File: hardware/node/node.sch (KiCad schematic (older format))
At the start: 64 parts, among them J1 BOOT0_Jumper, J2 FTDI, J3 SMA Female, J4 2 x AA, J5 SWD, Q1 Si2323DDS, SW1 TVCM04N016BB, U1 RFM69HW, U2 SHTC3, U3 AT25DF512C, U4 STM32L031K6Tx, Y1 32.768K-CFPX217

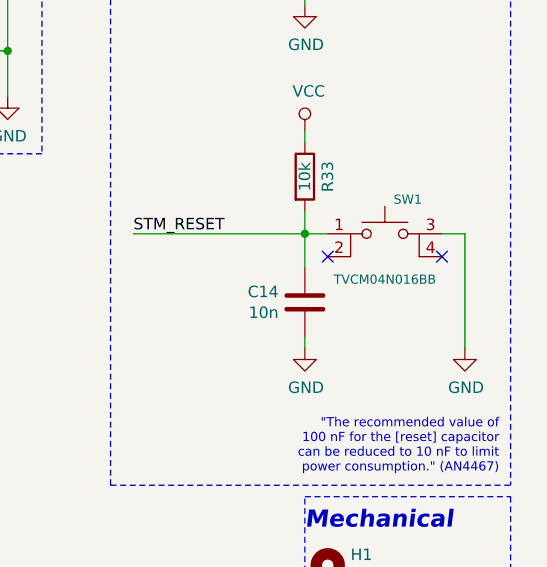
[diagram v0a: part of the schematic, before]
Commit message: Changed switch
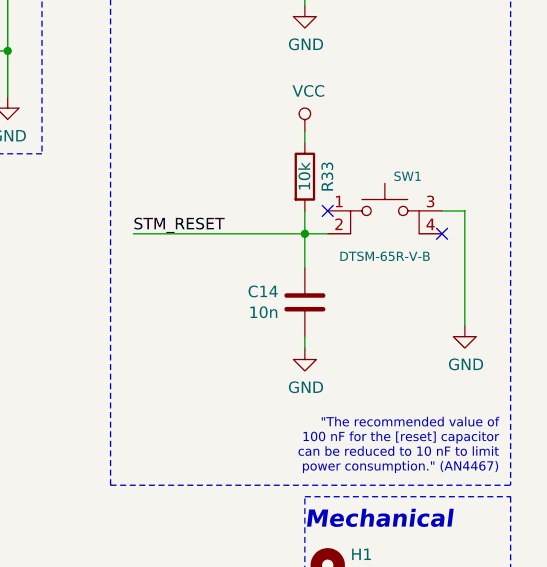
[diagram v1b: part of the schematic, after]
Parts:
- J2: footprint Connector_PinHeader_2.54mm:PinHeader_1x06_P2.54mm_Vertical -> Connector_PinHeader_2.54mm:PinHeader_1x06_P2.54mm_Horizontal
- SW1: value TVCM04N016BB -> DTSM-65R-V-B; footprint humidity:SW_TVCM04-N -> humidity:SW_SPST_DTSM-6
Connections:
- net STM_RESET: now also SW1.2; no longer SW1.1
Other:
- moved on the sheet: SW1
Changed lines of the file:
@@
 L power:GND #PWR032
 U 1 1 5CE4C513
-P 11000 3150
-F 0 "#PWR032" H 11000 2900 50  0001 C CNN
-F 1 "GND" H 11005 2977 50  0000 C CNN
-F 2 "" H 11000 3150 50  0001 C CNN
-F 3 "" H 11000 3150 50  0001 C CNN
-	1    11000 3150
-	1    0    0    -1
-$EndComp
-Wire Wire Line
-	10900 2650 11000 2650
-Wire Wire Line
-	11000 2650 11000 3150
+P 11000 3050
+F 0 "#PWR032" H 11000 2800 50  0001 C CNN
+F 1 "GND" H 11005 2877 50  0000 C CNN
+F 2 "" H 11000 3050 50  0001 C CNN
+F 3 "" H 11000 3050 50  0001 C CNN
+	1    11000 3050
+	1    0    0    -1
+$EndComp
+Wire Wire Line
+	10900 2550 11000 2550
+Wire Wire Line
+	11000 2550 11000 3050
 $Comp
 L Device:LED D2
@@
 F 0 "J2" H 4700 5100 50  0000 R CNN
 F 1 "FTDI" H 4700 4350 50  0000 C CNN
-F 2 "Connector_PinHeader_2.54mm:PinHeader_1x06_P2.54mm_Vertical" H 4600 4800 50  0001 C CNN
+F 2 "Connector_PinHeader_2.54mm:PinHeader_1x06_P2.54mm_Horizontal" H 4600 4800 50  0001 C CNN
 F 3 "~" H 4600 4800 50  0001 C CNN
 	1    4600 4800
@@
 L humidity:SW_Push_4pin SW1
 U 1 1 5DEFB807
-P 10650 2650
-F 0 "SW1" H 10750 2800 40  0000 C CNN
-F 1 "TVCM04N016BB" H 10650 2450 40  0000 C CNN
-F 2 "humidity:SW_TVCM04-N" H 10650 2650 40  0001 C CNN
-F 3 "https://www.tme.eu/Document/1590b299897e66d73e44ecd41b5c73b5/TVCM04N016BB.jpg" H 10650 2650 40  0001 C CNN
-	1    10650 2650
-	1    0    0    -1
-$EndComp
-NoConn ~ 10900 2750
-NoConn ~ 10400 2750
+P 10650 2550
+F 0 "SW1" H 10750 2700 40  0000 C CNN
+F 1 "DTSM-65R-V-B" H 10650 2350 40  0000 C CNN
+F 2 "humidity:SW_SPST_DTSM-6" H 10650 2550 40  0001 C CNN
+F 3 "https://www.tme.eu/se/en/details/dtsm-65r-v-b/microswitches-tact/diptronics/" H 10650 2550 40  0001 C CNN
+	1    10650 2550
+	1    0    0    -1
+$EndComp
+NoConn ~ 10900 2650
+NoConn ~ 10400 2550
 Text Notes 4100 7700 0    40   ~ 0
 Vary duty cycle linearly  depending\non VCC to get constant luminosity
